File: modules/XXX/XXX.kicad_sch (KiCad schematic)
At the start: 21 parts, among them J1 CardConnector, SW1 AS13AP, SW10 AS13AP, SW11 AS13AP, SW12 AS13AP, SW13 AS13AP, SW2 AS13AP, SW3 AS13AP, SW4 AS13AP, SW5 AS13AP, SW6 AS13AP, SW7 AS13AP, SW8 AS13AP, SW9 AS13AP

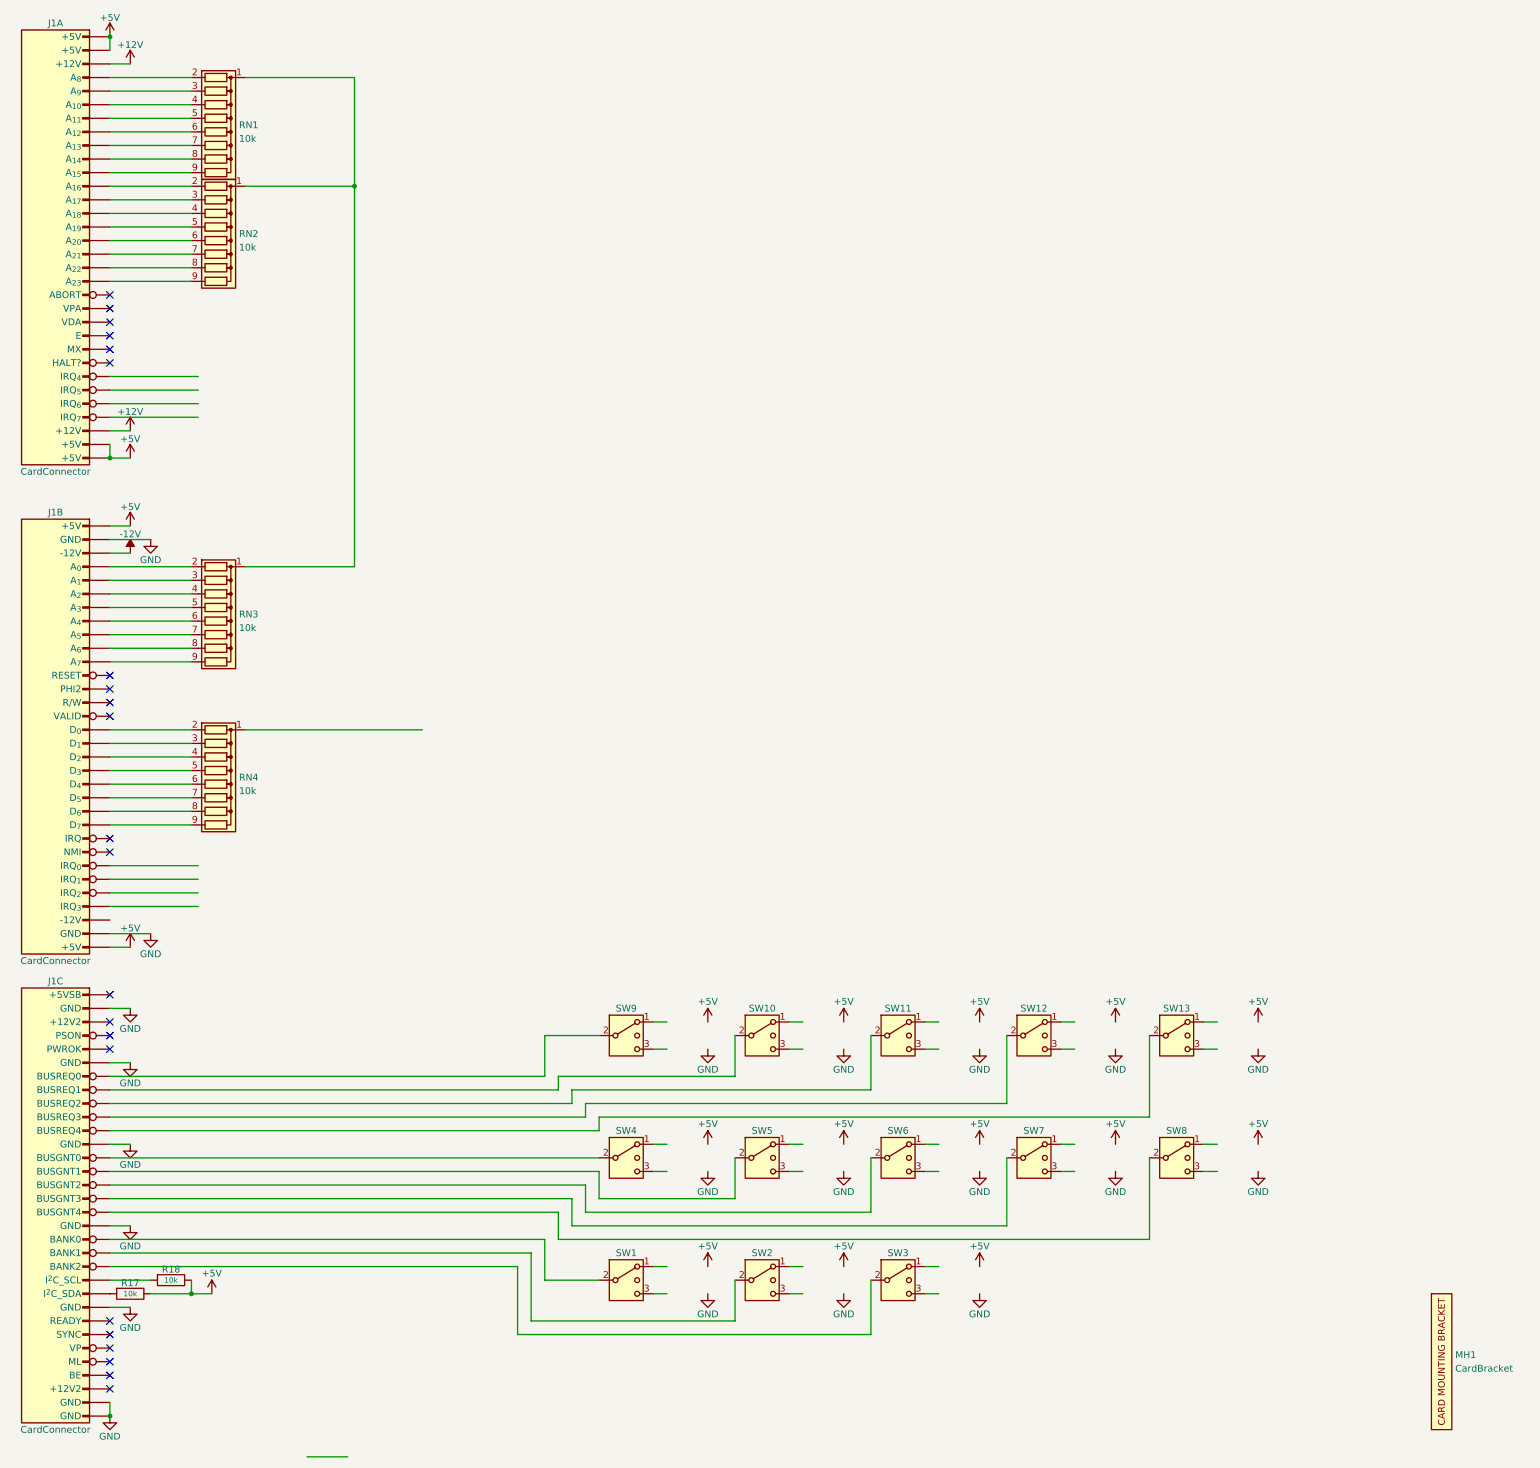
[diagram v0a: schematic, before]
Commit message: xxx bus terminator card
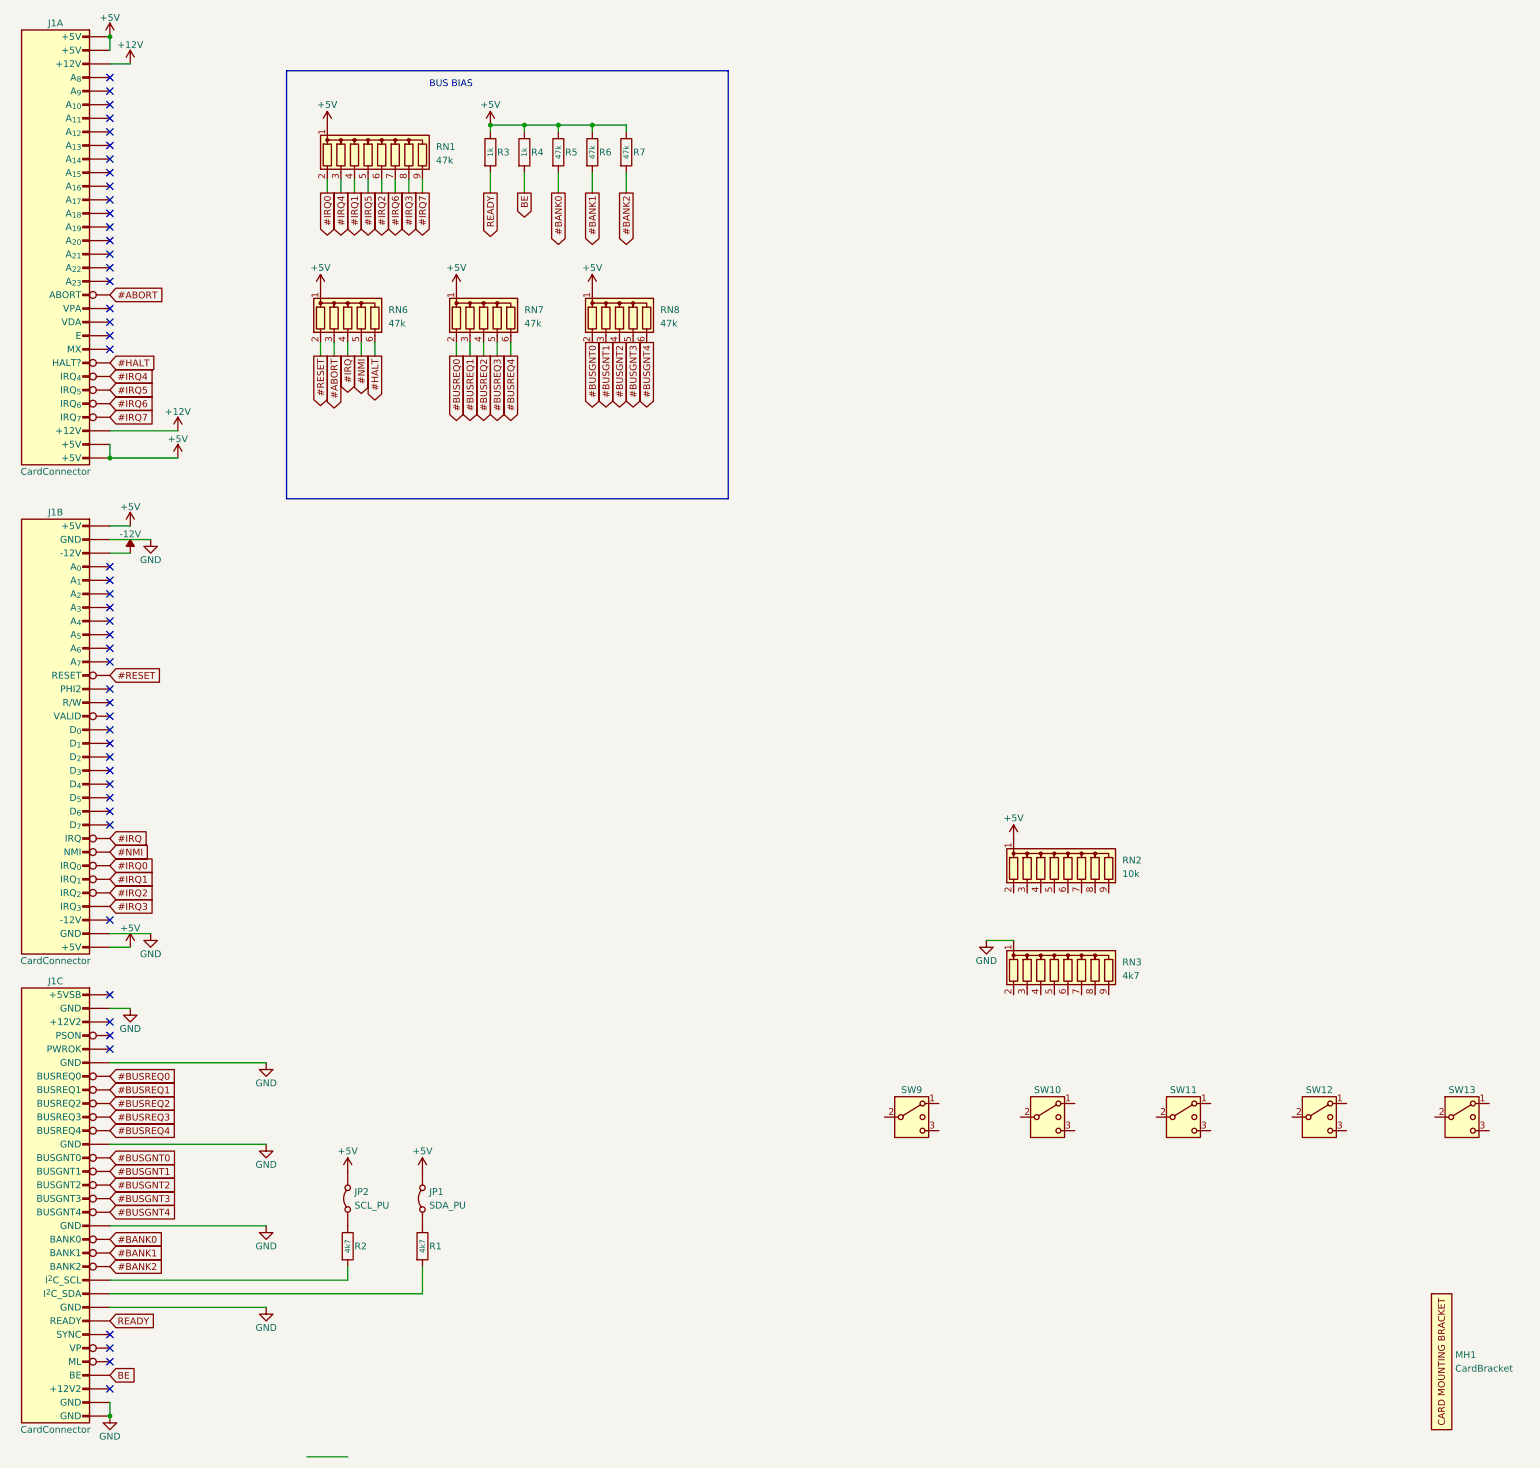
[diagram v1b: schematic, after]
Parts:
- removed R17, R18: 10k, IMNOTWOPR:R_Axial_DIN0207_P400mil, symbol IMNOTWOPR:R_Horizontal
- removed RN4: 10k, Resistor_THT:R_Array_SIP9, symbol Device:R_Network08
- removed SW1, SW2, SW3, SW4, SW5, SW6, SW7, SW8: AS13AP, IMNOTWOPR:AS13AP, symbol Switch:SW_SPDT_MSM
- added JP1: SDA_PU, IMNOTWOPR:Jumper_1x02, symbol Jumper:Jumper_2_Bridged
- added JP2: SCL_PU, IMNOTWOPR:Jumper_1x02, symbol Jumper:Jumper_2_Bridged
- added R1, R2: 4k7, IMNOTWOPR:R_Axial_DIN0207_P400mil, symbol IMNOTWOPR:R_Vertical
- added R3, R4: 1k, IMNOTWOPR:R_Axial_DIN0207_P400mil, symbol IMNOTWOPR:R_Vertical
- added R5, R6, R7: 47k, IMNOTWOPR:R_Axial_DIN0207_P400mil, symbol IMNOTWOPR:R_Vertical
- added RN6, RN7, RN8: 47k, Resistor_THT:R_Array_SIP6, symbol Device:R_Network05
- RN1: value 10k -> 47k
- RN3: value 10k -> 4k7
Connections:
- net +5V: now also RN1.1 (common), RN2.1 (common), JP1.2 (B), JP2.2 (B), R3.2, R4.2, R5.2, R6.2, R7.2, RN6.1 (common), RN7.1 (common), RN8.1 (common)
- net GND: now also RN3.1 (common)
- net at J1.b10 (A_{6}): no longer RN3.8 (R7)
- net at J1.b11 (A_{7}): no longer RN3.9 (R8)
- net #RESET: now reaches J1.b12 (RESET)
- net #RESET: now also RN6.2 (R1)
- net #IRQ: now reaches J1.b24 (IRQ)
- net #IRQ: now also RN6.4 (R3)
- net #NMI: now reaches J1.b25 (NMI)
- net #NMI: now also RN6.5 (R4)
- net #IRQ0: now reaches J1.b26 (IRQ_{0})
- net #IRQ0: now also RN1.2 (R1)
- net #IRQ1: now reaches J1.b27 (IRQ_{1})
- net #IRQ1: now also RN1.4 (R3)
- net #IRQ2: now reaches J1.b28 (IRQ_{2})
- net #IRQ2: now also RN1.6 (R5)
- net #IRQ3: now reaches J1.b29 (IRQ_{3})
- net #IRQ3: now also RN1.8 (R7)
- net at J1.b4 (A_{0}): no longer RN3.2 (R1)
- net at J1.b5 (A_{1}): no longer RN3.3 (R2)
- net at J1.b6 (A_{2}): no longer RN3.4 (R3)
- net at J1.b7 (A_{3}): no longer RN3.5 (R4)
- net at J1.b8 (A_{4}): no longer RN3.6 (R5)
- net at J1.b9 (A_{5}): no longer RN3.7 (R6)
- net #BANK1: now reaches J1.c20 (BANK1)
- net #BANK1: now also R6.1
- net #BUSGNT1: now reaches J1.c14 (BUSGNT1)
- net #BUSGNT1: now also RN8.3 (R2)
- net at J1.a4 (A_{8}): no longer RN1.2 (R1)
- net at J1.a5 (A_{9}): no longer RN1.3 (R2)
- net at J1.a6 (A_{10}): no longer RN1.4 (R3)
- net at J1.a7 (A_{11}): no longer RN1.5 (R4)
- net at J1.a8 (A_{12}): no longer RN1.6 (R5)
- net at J1.a9 (A_{13}): no longer RN1.7 (R6)
- net at J1.a10 (A_{14}): no longer RN1.8 (R7)
- net at J1.a11 (A_{15}): no longer RN1.9 (R8)
- net #BUSGNT4: now reaches J1.c17 (BUSGNT4)
- net #BUSGNT4: now also RN8.6 (R5)
- net at J1.a12 (A_{16}): no longer RN2.2 (R1)
- net at J1.a13 (A_{17}): no longer RN2.3 (R2)
- net at J1.a14 (A_{18}): no longer RN2.4 (R3)
- net at J1.a15 (A_{19}): no longer RN2.5 (R4)
- net at J1.a16 (A_{20}): no longer RN2.6 (R5)
- net at J1.a17 (A_{21}): no longer RN2.7 (R6)
- net at J1.a18 (A_{22}): no longer RN2.8 (R7)
- net at J1.a19 (A_{23}): no longer RN2.9 (R8)
- net #ABORT: now reaches J1.a20 (ABORT)
- net #ABORT: now also RN6.3 (R2)
- net #HALT: now reaches J1.a25 (HALT?)
- net #HALT: now also RN6.6 (R5)
- net #IRQ4: now reaches J1.a26 (IRQ_{4})
- net #IRQ4: now also RN1.3 (R2)
- net #IRQ5: now reaches J1.a27 (IRQ_{5})
- net #IRQ5: now also RN1.5 (R4)
- net #IRQ6: now reaches J1.a28 (IRQ_{6})
- net #IRQ6: now also RN1.7 (R6)
- net #IRQ7: now reaches J1.a29 (IRQ_{7})
- net #IRQ7: now also RN1.9 (R8)
- net #BUSGNT0: now reaches J1.c13 (BUSGNT0)
- net #BUSGNT0: now also RN8.2 (R1)
- net at SW12.2 (3): no longer J1.c10 (BUSREQ3)
- net at SW10.2 (3): no longer J1.c8 (BUSREQ1)
- net at J1.c22 (I^{2}C_SCL): now also R2.1
- net at SW13.2 (3): no longer J1.c11 (BUSREQ4)
- net at J1.c23 (I^{2}C_SDA): now also R1.1
- net #BANK2: now reaches J1.c21 (BANK2)
- net #BANK2: now also R7.1
- net #BUSGNT2: now reaches J1.c15 (BUSGNT2)
- net #BUSGNT2: now also RN8.4 (R3)
- net at SW11.2 (3): no longer J1.c9 (BUSREQ2)
- net #BANK0: now reaches J1.c19 (BANK0)
- net #BANK0: now also R5.1
- net #BUSGNT3: now reaches J1.c16 (BUSGNT3)
- net #BUSGNT3: now also RN8.5 (R4)
- net READY: now reaches J1.c25 (READY)
- net READY: now also R3.1
- net BE: now reaches J1.c29 (BE)
- net BE: now also R4.1
- net at SW9.2 (3): no longer J1.c7 (BUSREQ0)
- new net: JP2.1 (A), R2.2
- new net: JP1.1 (A), R1.2
- new net #BUSREQ0: J1.c7 (BUSREQ0), RN7.2 (R1)
- new net #BUSREQ1: J1.c8 (BUSREQ1), RN7.3 (R2)
- new net #BUSREQ2: J1.c9 (BUSREQ2), RN7.4 (R3)
- new net #BUSREQ3: J1.c10 (BUSREQ3), RN7.5 (R4)
- new net #BUSREQ4: J1.c11 (BUSREQ4), RN7.6 (R5)
- no-connect marks 22 -> 48
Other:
- note added: "BUS BIAS"
- moved on the sheet: SW10, SW11, SW12, SW13, SW9
